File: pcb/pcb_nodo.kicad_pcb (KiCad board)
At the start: 2 copper layers, 101 x 48 mm, 26 parts, among them J1 Conn_01x02, J2 Conn_01x02, J3 Conn_01x03, J4 Conn_01x04, J5 Conn_01x18, J6 Conn_01x18, J7 UART_0, K1 FINDER-36.11, Q1 2N2219, Q2 2N2219, SW1 SW_Push, SW2 SW_Push, U1 DHT11

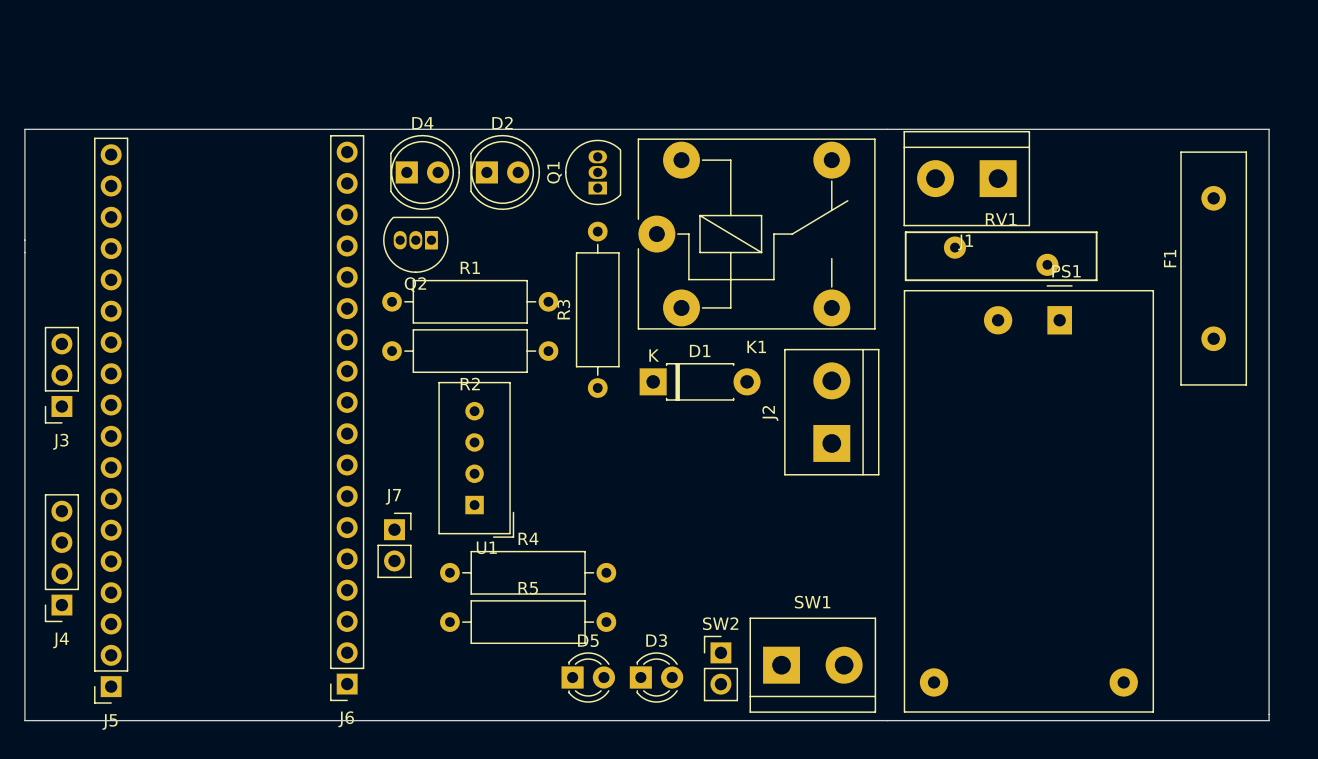
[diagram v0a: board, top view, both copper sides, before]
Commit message: enrutado
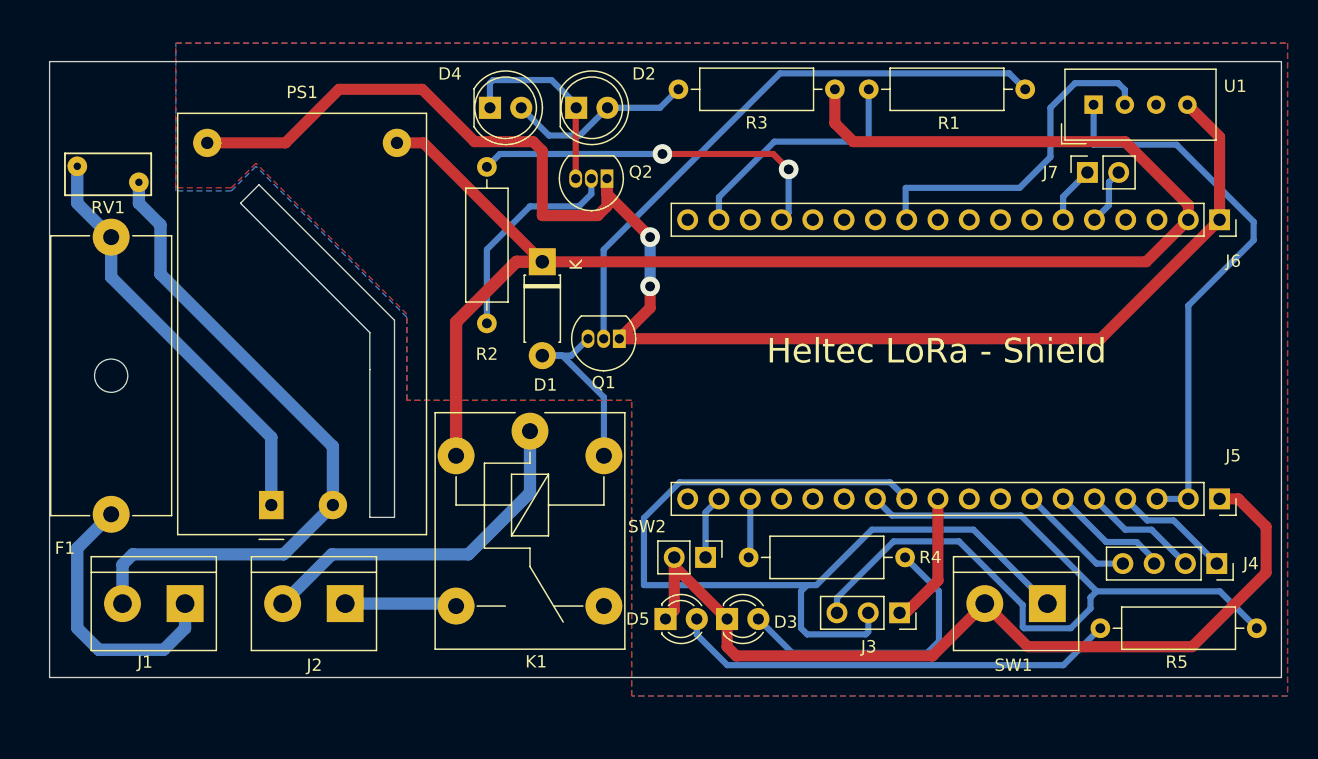
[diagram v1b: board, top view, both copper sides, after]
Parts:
- F1: footprint Fuse:Fuse_Littelfuse-LVR100 -> Fuse:Fuseholder_Cylinder-5x20mm_Schurter_0031_8201_Horizontal_Open
- RV1: footprint Varistor:RV_Disc_D15.5mm_W3.9mm_P7.5mm -> Varistor:RV_Disc_D7mm_W3.4mm_P5mm
- moved J4 93.8 mm to (144.8, 70.8), turned to 270 degrees
- moved J5 91.3 mm to (145.0, 65.5), turned to 270 degrees
- moved F1 89.9 mm to (55.0, 44.2), turned to 270 degrees
- moved J6 80.2 mm to (145.0, 42.8), turned to 270 degrees
- moved RV1 79.2 mm to (52.2, 38.5), turned to 0 degrees
- moved J1 74.5 mm to (61.0, 74.0)
- moved J3 70.0 mm to (119.0, 74.8), turned to 270 degrees
- moved PS1 65.7 mm to (68.0, 66.0), turned to 90 degrees
- moved R5 65.5 mm to (148.0, 76.0), turned to 180 degrees
- moved J7 63.3 mm to (134.2, 39.0), turned to 90 degrees
- moved U1 59.8 mm to (134.8, 33.5), turned to 90 degrees
- moved R1 42.4 mm to (116.5, 32.2)
- moved J2 41.6 mm to (74.0, 74.0), turned to 180 degrees
- moved R3 31.0 mm to (113.8, 32.2), turned to 180 degrees
- moved R4 24.3 mm to (106.8, 70.2)
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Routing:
- net GND: track 0.00 -> 195.3 mm, vias 0 -> 2
- net +5V: track 0.00 -> 124.9 mm
- net /33: track 0.00 -> 76.6 mm
- net /25: track 0.00 -> 65.2 mm
- net Net-(J1-Pad2): track 0.00 -> 55.0 mm
- net Net-(Q1-Pad2): track 0.00 -> 47.9 mm
- net +3V3: track 0.00 -> 46.1 mm
- net Net-(D5-Pad2): track 0.00 -> 36.3 mm
- net Net-(F1-Pad1): track 0.00 -> 34.0 mm
- net /2: track 0.00 -> 29.8 mm, vias 0 -> 2
- net Net-(J2-Pad2): track 0.00 -> 28.8 mm
- net /23: track 0.00 -> 27.7 mm
- net Net-(D3-Pad2): track 0.00 -> 24.1 mm
- net Net-(F1-Pad2): track 0.00 -> 22.6 mm
- net /17: track 0.00 -> 20.1 mm
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- added copper zone on B.Cu, net GND
- added copper zone on F.Cu, net GND
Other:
- board size 101 x 48 mm -> 100 x 50 mm
- net class Default: clearance 0.8 -> 0.25
- rule trace_clearance: 0.8 -> 0.25
- board text added: "Heltec LoRa - Shield"
- board text removed: "SPB - Lucas ML"

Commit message: avances
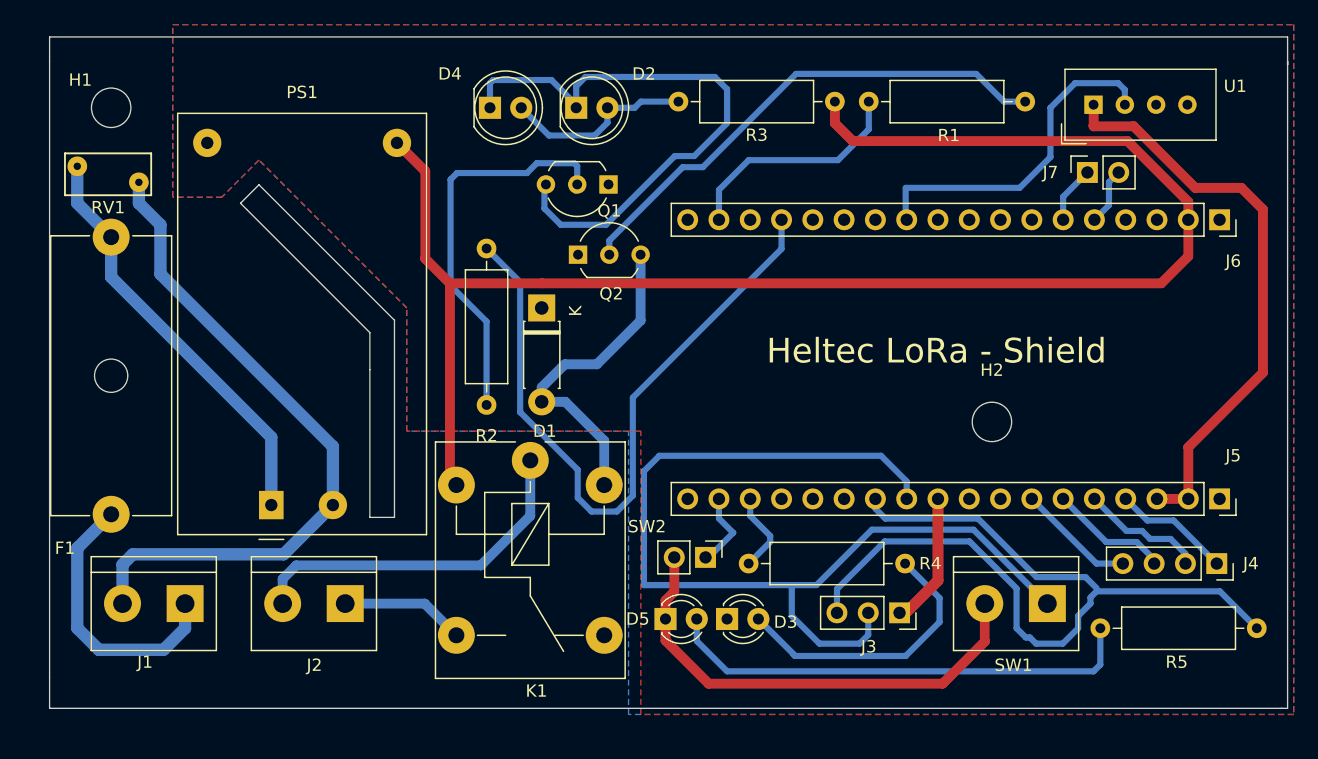
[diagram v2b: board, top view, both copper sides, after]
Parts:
- added H1: MountingHole_3.2mm_M3, MountingHole:MountingHole_3.2mm_M3, F.Cu at (55.0, 33.8)
- added H2: MountingHole_3.2mm_M3, MountingHole:MountingHole_3.2mm_M3, F.Cu at (126.5, 59.2)
- Q1, Q2: footprint Package_TO_SOT_THT:TO-92_Inline -> Package_TO_SOT_THT:TO-92_Inline_Wide
- moved Q1 7.60 mm to (92.9, 45.7), turned to 0 degrees
- moved R2 6.63 mm to (85.5, 57.9)
- moved D1 3.75 mm to (90.0, 50.0)
- moved K1 2.38 mm to (89.0, 62.4)
- moved R1 1.00 mm to (116.5, 33.2)
- moved R3 1.00 mm to (113.8, 33.2)
- moved R4 0.50 mm to (106.8, 70.8)
- moved Q2 0.49 mm to (95.4, 40.0)
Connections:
- net /12 renamed /led1
- net /13 renamed /pulsador2
- net /17 renamed /salidarelay
- net /2 renamed /salidair
- net /23 renamed /temp
- net /25 renamed /led2
- net /33 renamed /pulsador1
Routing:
- net GND: track 195.3 -> 38.9 mm, vias 2 -> 0
- net Net-(D2-Pad1): track 15.9 -> 48.5 mm
- net /salidair: track 29.8 -> 56.2 mm, vias 2 -> 0
- net Net-(Q2-Pad2): track 17.6 -> 32.0 mm
- net Net-(D1-Pad2): track 15.4 -> 26.8 mm
- net Net-(Q1-Pad2): track 47.9 -> 41.4 mm
- net /pulsador1: track 76.6 -> 82.2 mm
- net +5V: track 124.9 -> 128.1 mm
- net /led2: track 65.2 -> 68.2 mm
- net Net-(D5-Pad2): track 36.3 -> 38.7 mm
- net /led1: track 4.80 -> 6.65 mm
- net /salidarelay: track 20.1 -> 18.9 mm
- net /pulsador2: track 5.20 -> 6.31 mm
- net Net-(D3-Pad2): track 24.1 -> 23.0 mm
- net Net-(J2-Pad1): track 9.08 -> 10.1 mm
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- added copper zone on F.Cu, net +5V
- removed copper zone on F.Cu, net GND
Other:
- board size 100 x 50 mm -> 100.5 x 54.5 mm
- net class Default: clearance 0.25 -> 0.4
- rule trace_clearance: 0.25 -> 0.4
- rule via_min_size: 0.4 -> 0.5
